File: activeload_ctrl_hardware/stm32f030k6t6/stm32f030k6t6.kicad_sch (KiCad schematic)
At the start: 43 parts

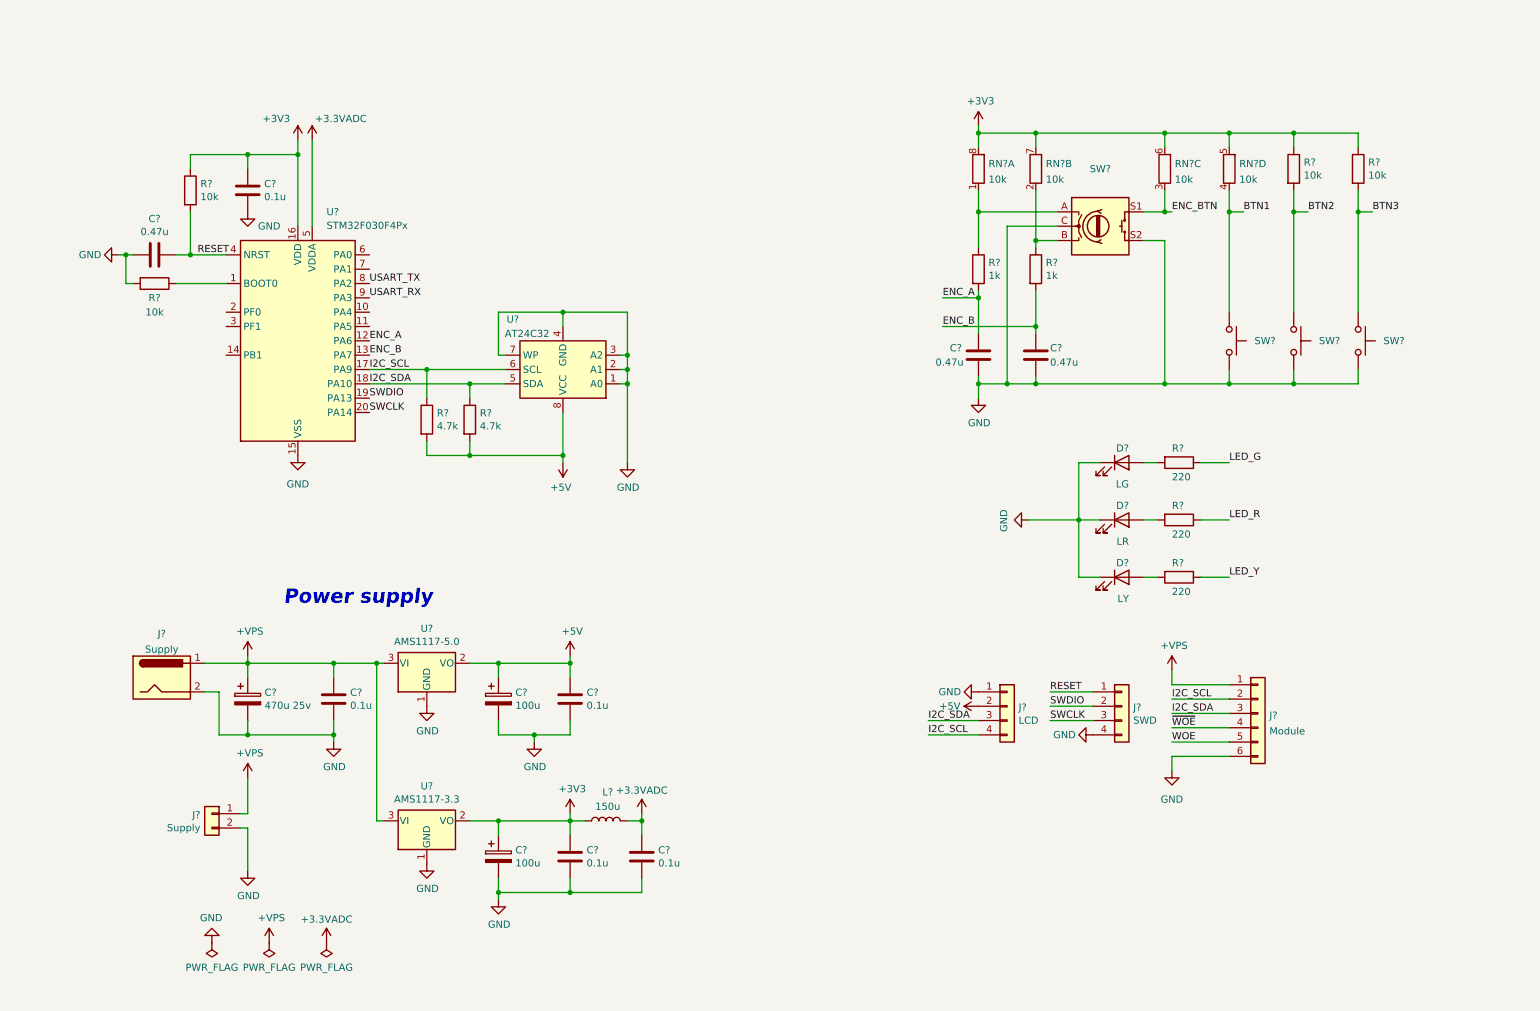
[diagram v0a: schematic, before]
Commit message: stm32f0k6t6 scheme
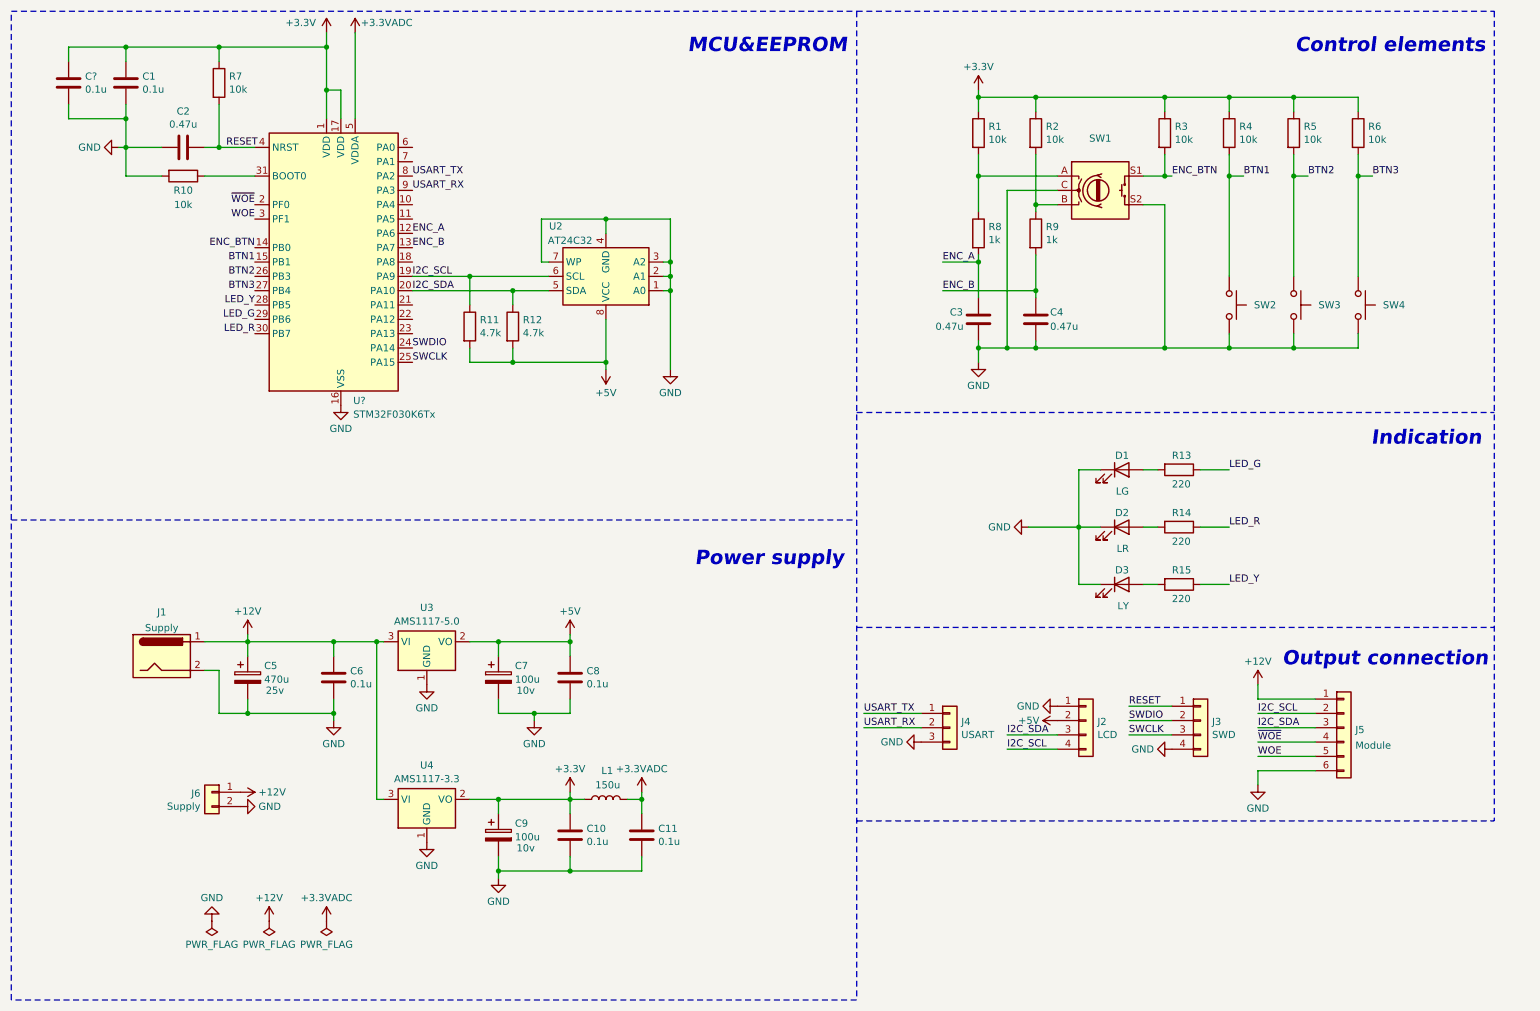
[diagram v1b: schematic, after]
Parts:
- removed C? (x2): 100u, Capacitor_THT:CP_Radial_D4.0mm_P2.00mm, symbol Device:CP
- removed C?: 470u 25v, Capacitor_THT:C_Radial_D8.0mm_H7.0mm_P3.50mm, symbol Device:CP
- removed R?: 10k, Resistor_SMD:R_1206_3216Metric_Pad1.30x1.75mm_HandSolder, symbol Device:R
- removed RN? (x4): 10k, Resistor_SMD:R_Array_Convex_4x1206, symbol Device:R_Pack04_Split
- removed SW?: (no value), Rotary_Encoder:RotaryEncoder_Alps_EC12E-Switch_Vertical_H20mm, symbol Device:Rotary_Encoder_Switch
- removed U?: AMS1117-5.0, Package_TO_SOT_SMD:SOT-223-3_TabPin2, symbol Regulator_Linear:AMS1117-5.0
- removed U?: STM32F030F4Px, Package_SO:TSSOP-20_4.4x6.5mm_P0.65mm, symbol MCU_ST_STM32F0:STM32F030F4Px
- removed U?: AMS1117-3.3, Package_TO_SOT_SMD:SOT-223-3_TabPin2, symbol Regulator_Linear:AMS1117-3.3
- added C5: 470u, Capacitor_THT:C_Radial_D8.0mm_H7.0mm_P3.50mm, symbol Device:C_Polarized
- added C7, C9: 100u, Capacitor_THT:CP_Radial_D4.0mm_P2.00mm, symbol Device:C_Polarized
- added C?: 0.1u, Capacitor_SMD:C_0805_2012Metric_Pad1.18x1.45mm_HandSolder, symbol Device:C
- added J4: USART, Connector_PinHeader_2.54mm:PinHeader_1x03_P2.54mm_Vertical, symbol Connector_Generic:Conn_01x03
- added R1, R2, R3, R4, R5: 10k, Resistor_SMD:R_1206_3216Metric_Pad1.30x1.75mm_HandSolder, symbol Device:R
- added SW1: ~, Rotary_Encoder:RotaryEncoder_Alps_EC12E-Switch_Vertical_H20mm, symbol Device:RotaryEncoder_Switch
- added U3: AMS1117-5.0, Package_TO_SOT_SMD:SOT-223-3_TabPin2, symbol Regulator_Linear:AMS1117-5.0
- added U4: AMS1117-3.3, Package_TO_SOT_SMD:SOT-223-3_TabPin2, symbol Regulator_Linear:AMS1117-3.3
- added U?: STM32F030K6Tx, Package_QFP:LQFP-32_7x7mm_P0.8mm, symbol MCU_ST_STM32F0:STM32F030K6Tx
- gave numbers to parts that had none: 31
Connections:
- net +3.3VADC: now also U?.5 (VDDA)
- net +5V: now also C7.1, U3.2 (VO)
- net BTN1: now also R4.2, U?.15 (PB1)
- net BTN2: now also R5.2, U?.26 (PB3)
- net BTN3: now also U?.27 (PB4)
- net ENC_A: now also U?.12 (PA6)
- net ENC_B: now also U?.13 (PA7)
- net ENC_BTN: now also R3.2, SW1.S1, U?.14 (PB0)
- net GND: now also C5.2, C7.2, C9.2, C?.2, J4.3 (Pin_3), SW1.C, SW1.S2, U3.1 (GND), U4.1 (GND), U?.16 (VSS), U?.32 (VSS)
- net I2C_SCL: now also U?.19 (PA9)
- net I2C_SDA: now also U?.20 (PA10)
- net LED_G: now also U?.29 (PB6)
- net LED_R: now also U?.30 (PB7)
- net LED_Y: now also U?.28 (PB5)
- net RESET: now also U?.4 (NRST)
- net SWCLK: now also U?.25 (PA15)
- net SWDIO: now also U?.24 (PA14)
- net USART_RX: now also J4.2 (Pin_2), U?.9 (PA3)
- net USART_TX: now also J4.1 (Pin_1), U?.8 (PA2)
- net WOE: now also U?.3 (PF1)
- net ~{WOE}: now also U?.2 (PF0)
- net at R8.1: now also R1.2, SW1.A
- net at R10.1: now also U?.31 (BOOT0)
- net at R9.1: now also R2.2, SW1.B
- net +3V3 renamed +3.3V
- net +3.3V: now also C9.1, C?.1, R1.1, R2.1, R3.1, R4.1, R5.1, U4.2 (VO), U?.1 (VDD), U?.17 (VDD)
- net +VPS renamed +12V
- net +12V: now also C5.1, U3.3 (VI), U4.3 (VI)
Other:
- note added: "Control elements"
- note added: "Indication"
- note added: "MCU&EEPROM"
- note added: "Output connection"
- moved on the sheet: C1, C10, C11, C2, C3, C4, C6, C8, D1, D2, D3, J1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
